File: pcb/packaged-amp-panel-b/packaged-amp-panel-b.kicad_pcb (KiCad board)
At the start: 2 copper layers, 60 x 22.7 mm, 1 part

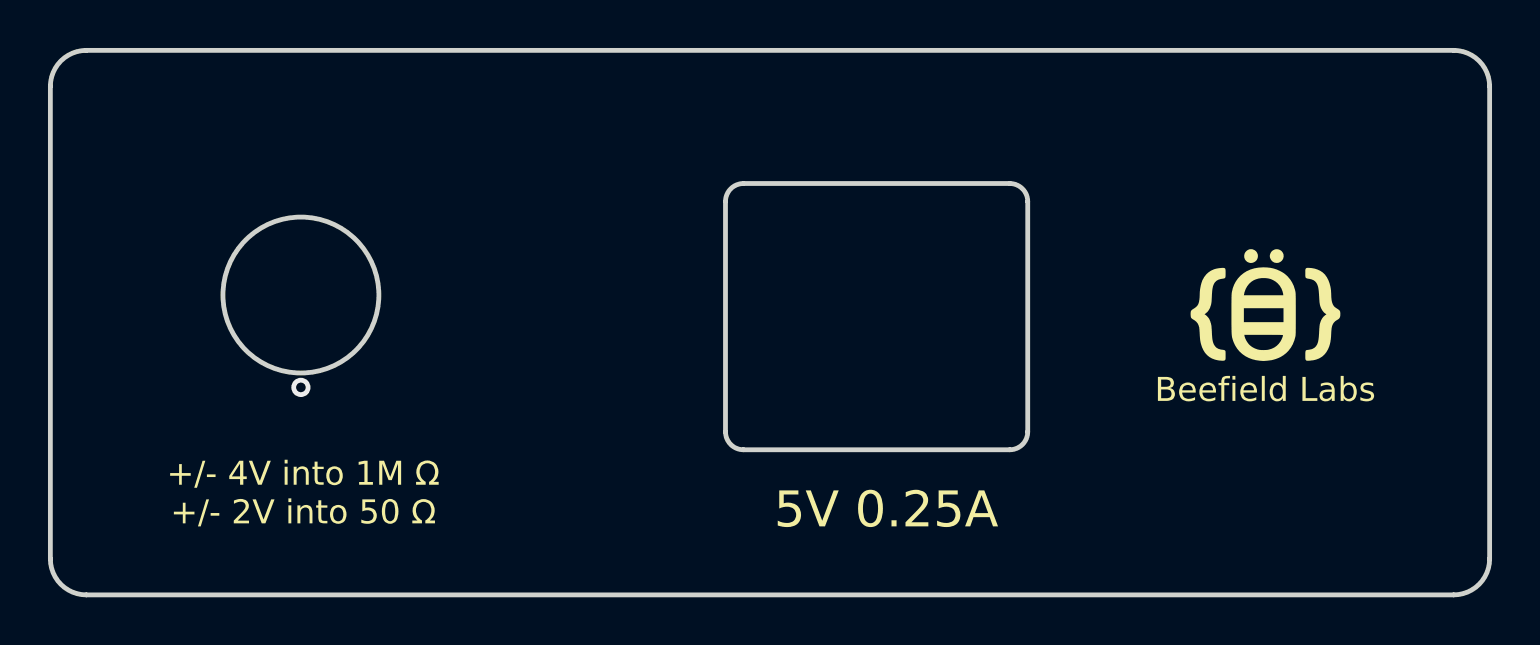
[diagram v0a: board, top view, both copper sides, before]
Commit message: next revision
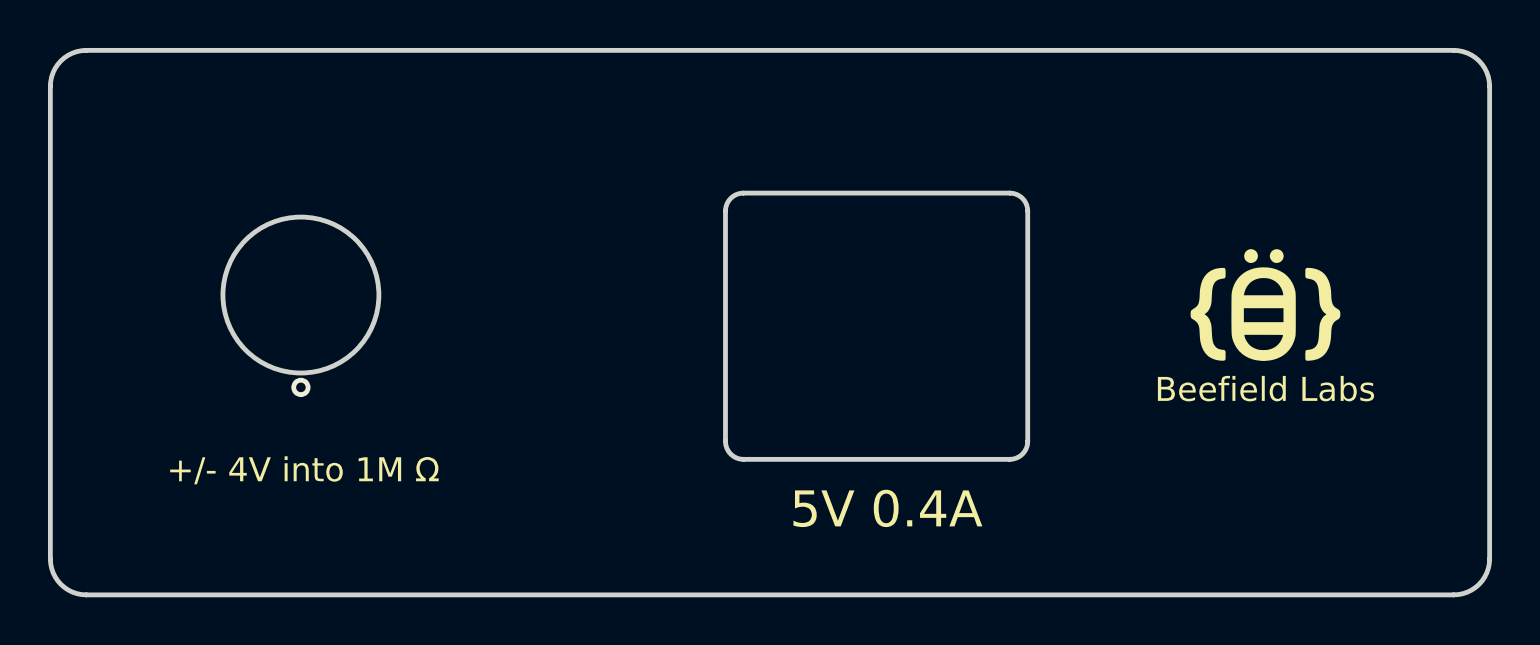
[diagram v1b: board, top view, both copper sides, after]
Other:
- outline, holes or cut-outs redrawn
- board text added: "+/- 4V into 1M Ω"
- board text added: "5V 0.4A"
- board text removed: "+/- 4V into 1M Ω +/- 2V into 50 Ω"
- board text removed: "5V 0.25A"
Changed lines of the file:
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@@
   (gr_line (start 152.555626 58.25) (end 95.555626 58.25) (layer "Edge.Cuts") (width 0.2))
   (gr_arc (start 95.555626 80.95) (mid 94.494966 80.51066) (end 94.055626 79.45) (layer "Edge.Cuts") (width 0.2))
-  (gr_line (start 122.95 63.8) (end 134.05 63.8) (layer "Edge.Cuts") (width 0.2))
-  (gr_line (start 134.8 64.55) (end 134.8 74.15) (layer "Edge.Cuts") (width 0.2))
-  (gr_arc (start 122.2 64.55) (mid 122.41967 64.01967) (end 122.95 63.8) (layer "Edge.Cuts") (width 0.2))
+  (gr_line (start 122.95 64.2) (end 134.05 64.2) (layer "Edge.Cuts") (width 0.2))
+  (gr_line (start 134.8 64.95) (end 134.8 74.55) (layer "Edge.Cuts") (width 0.2))
+  (gr_arc (start 122.2 64.95) (mid 122.41967 64.41967) (end 122.95 64.2) (layer "Edge.Cuts") (width 0.2))
   (gr_line (start 95.555626 80.95) (end 152.555626 80.95) (layer "Edge.Cuts") (width 0.2))
   (gr_line (start 94.055626 59.75) (end 94.055626 79.45) (layer "Edge.Cuts") (width 0.2))
-  (gr_line (start 122.2 74.15) (end 122.2 64.55) (layer "Edge.Cuts") (width 0.2))
-  (gr_arc (start 134.05 63.8) (mid 134.580347 64.019661) (end 134.8 64.55) (layer "Edge.Cuts") (width 0.2))
-  (gr_arc (start 134.8 74.15) (mid 134.580329 74.680321) (end 134.05 74.9) (layer "Edge.Cuts") (width 0.2))
+  (gr_line (start 122.2 74.55) (end 122.2 64.95) (layer "Edge.Cuts") (width 0.2))
+  (gr_arc (start 134.05 64.2) (mid 134.58033 64.41967) (end 134.8 64.95) (layer "Edge.Cuts") (width 0.2))
+  (gr_arc (start 134.8 74.55) (mid 134.58033 75.08033) (end 134.05 75.3) (layer "Edge.Cuts") (width 0.2))
   (gr_arc (start 154.055626 79.45) (mid 153.616286 80.51066) (end 152.555626 80.95) (layer "Edge.Cuts") (width 0.2))
-  (gr_arc (start 122.95 74.9) (mid 122.41967 74.68033) (end 122.2 74.15) (layer "Edge.Cuts") (width 0.2))
+  (gr_arc (start 122.95 75.3) (mid 122.41967 75.08033) (end 122.2 74.55) (layer "Edge.Cuts") (width 0.2))
   (gr_arc (start 152.555626 58.25) (mid 153.616286 58.68934) (end 154.055626 59.75) (layer "Edge.Cuts") (width 0.2))
-  (gr_line (start 134.05 74.9) (end 122.95 74.9) (layer "Edge.Cuts") (width 0.2))
+  (gr_line (start 134.05 75.3) (end 122.95 75.3) (layer "Edge.Cuts") (width 0.2))
   (gr_circle (center 104.5 68.45) (end 107.75 68.45) (layer "Edge.Cuts") (width 0.2) (fill none))
   (gr_arc (start 94.055626 59.75) (mid 94.494966 58.68934) (end 95.555626 58.25) (layer "Edge.Cuts") (width 0.2))
@@
     (effects (font (size 1 1) (thickness 0.15)))
   )
-  (gr_text "+/- 4V into 1M Ω\n+/- 2V into 50 Ω" (at 104.6 76.7) (layer "F.SilkS")
+  (gr_text "+/- 4V into 1M Ω\n" (at 104.6 75.75) (layer "F.SilkS")
     (effects (font (size 1 1) (thickness 0.15)))
   )
-  (gr_text "5V 0.25A" (at 128.9 77.4) (layer "F.SilkS")
+  (gr_text "5V 0.4A" (at 128.9 77.4) (layer "F.SilkS")
     (effects (font (size 1.5 1.5) (thickness 0.3)))
   )
   (via (at 104.5 72.3) (size 0.8) (drill 0.4) (layers "F.Cu" "B.Cu") (free) (net 0))
-  (group "" (id f9fdcc45-efb5-407b-b873-9a2d7f0315bf)
-    (members
-      07d800d4-d1db-46ff-ae85-79cface2e4d4
-      0cdfe85b-4f6e-4881-ae9b-b3a882345efb
-      0ddb953f-205f-442b-b848-cf6a84317acc
-      3ecff5c9-24c9-4b4c-91e3-d4a830dd4dd0
-      40e926c5-3a86-445a-9f98-5d4e13723fc0
-      5358da93-8fd2-4dae-9497-ff676879ac9e
-      758d1bd0-f422-43f7-91fd-b4af91de7a5b
-      8144efa2-cec2-46cd-8eab-3e82ee343a28
-      8cc84535-8f6b-4ccb-b4cf-62f6cd0d6d7e
-      97031a12-d7c5-4715-afb1-3668add88d16
-      98678171-d971-4195-bd43-daab671d4ca8
-      9c24e488-9c8d-49b2-9078-ea3751022922
-      a7e9c2fe-3664-4278-9084-35ef16da3316
-      c01e6209-d77a-466c-bdb7-680bf35e795a
-      d7eaec30-a976-4998-a849-895c3e24c2d4
-      f952d511-d473-4134-9274-6869ab0e1b67
-      ff6fc7e0-808d-45fd-aa64-d0c7724f8d98
-    )
-  )
 )
